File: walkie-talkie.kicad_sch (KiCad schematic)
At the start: 15 parts, among them J1 I2C, J2 Conn_01x08, J3 esp32-pico-kit, SW1 Transmit, SW2 POWER, U1 WARNING: Switch off when Plug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, U2 adafruit-MAX98357, U3 mems-mic

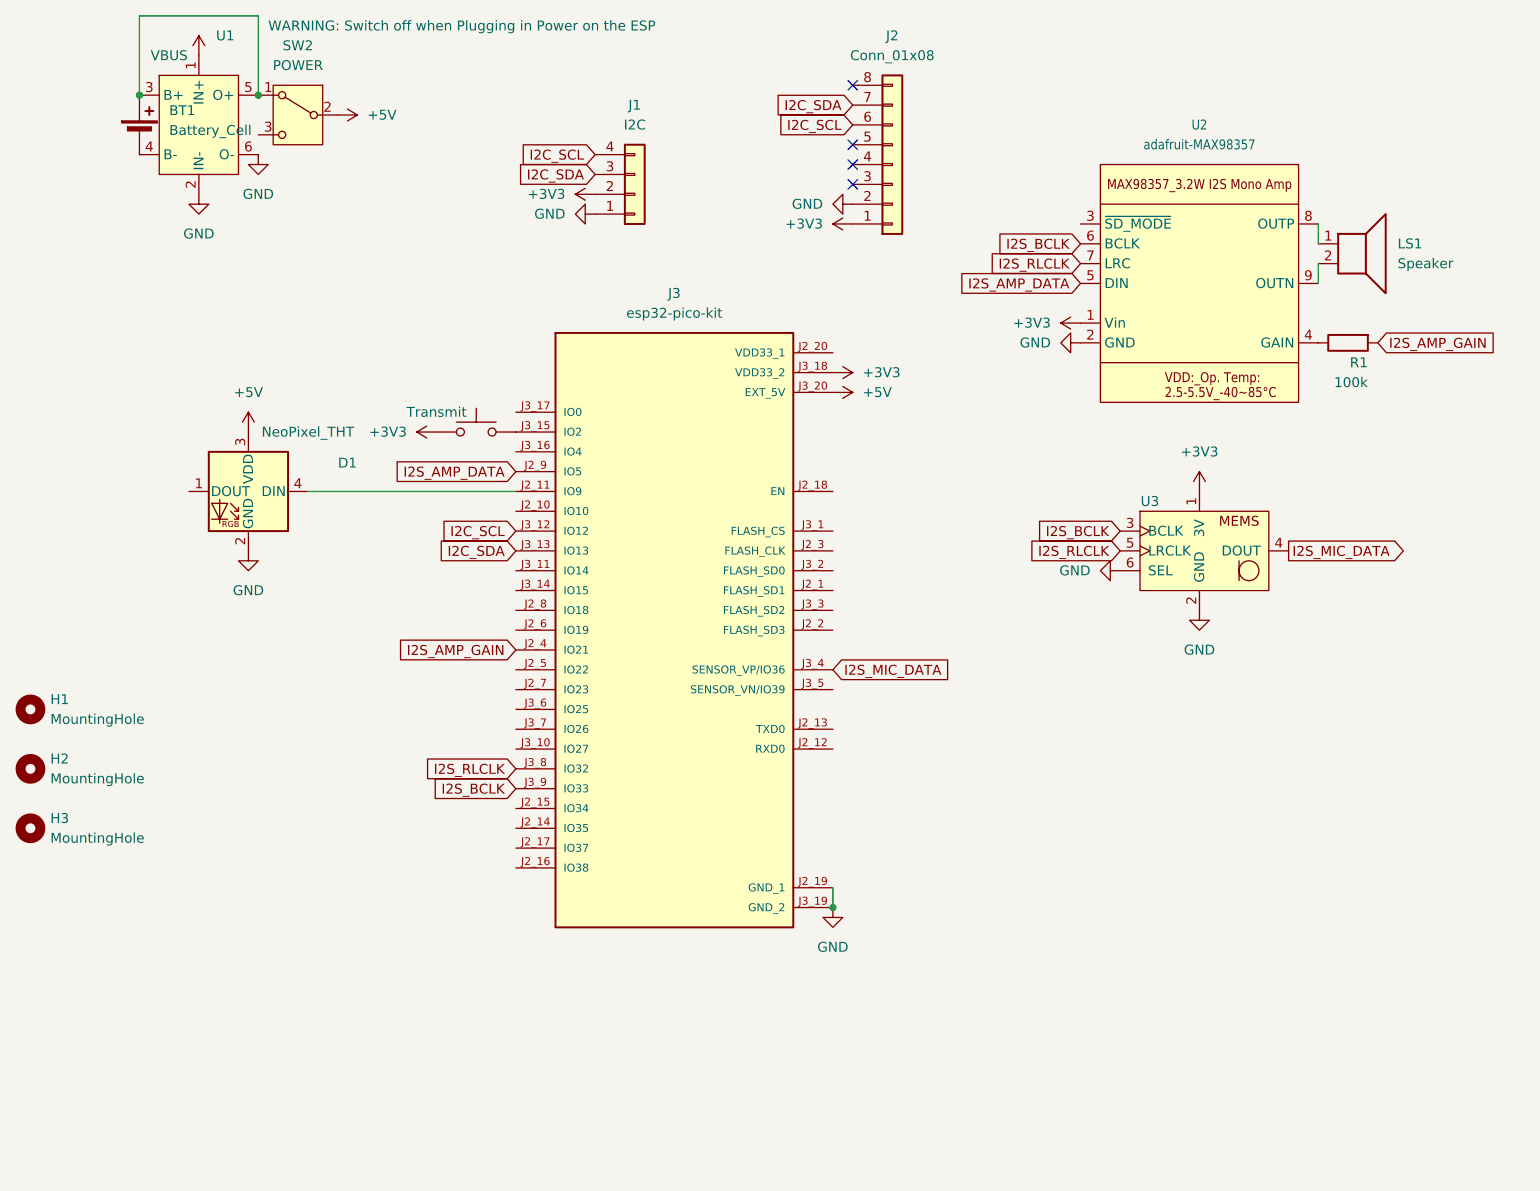
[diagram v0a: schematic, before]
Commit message: Lolin32-Lite PCB
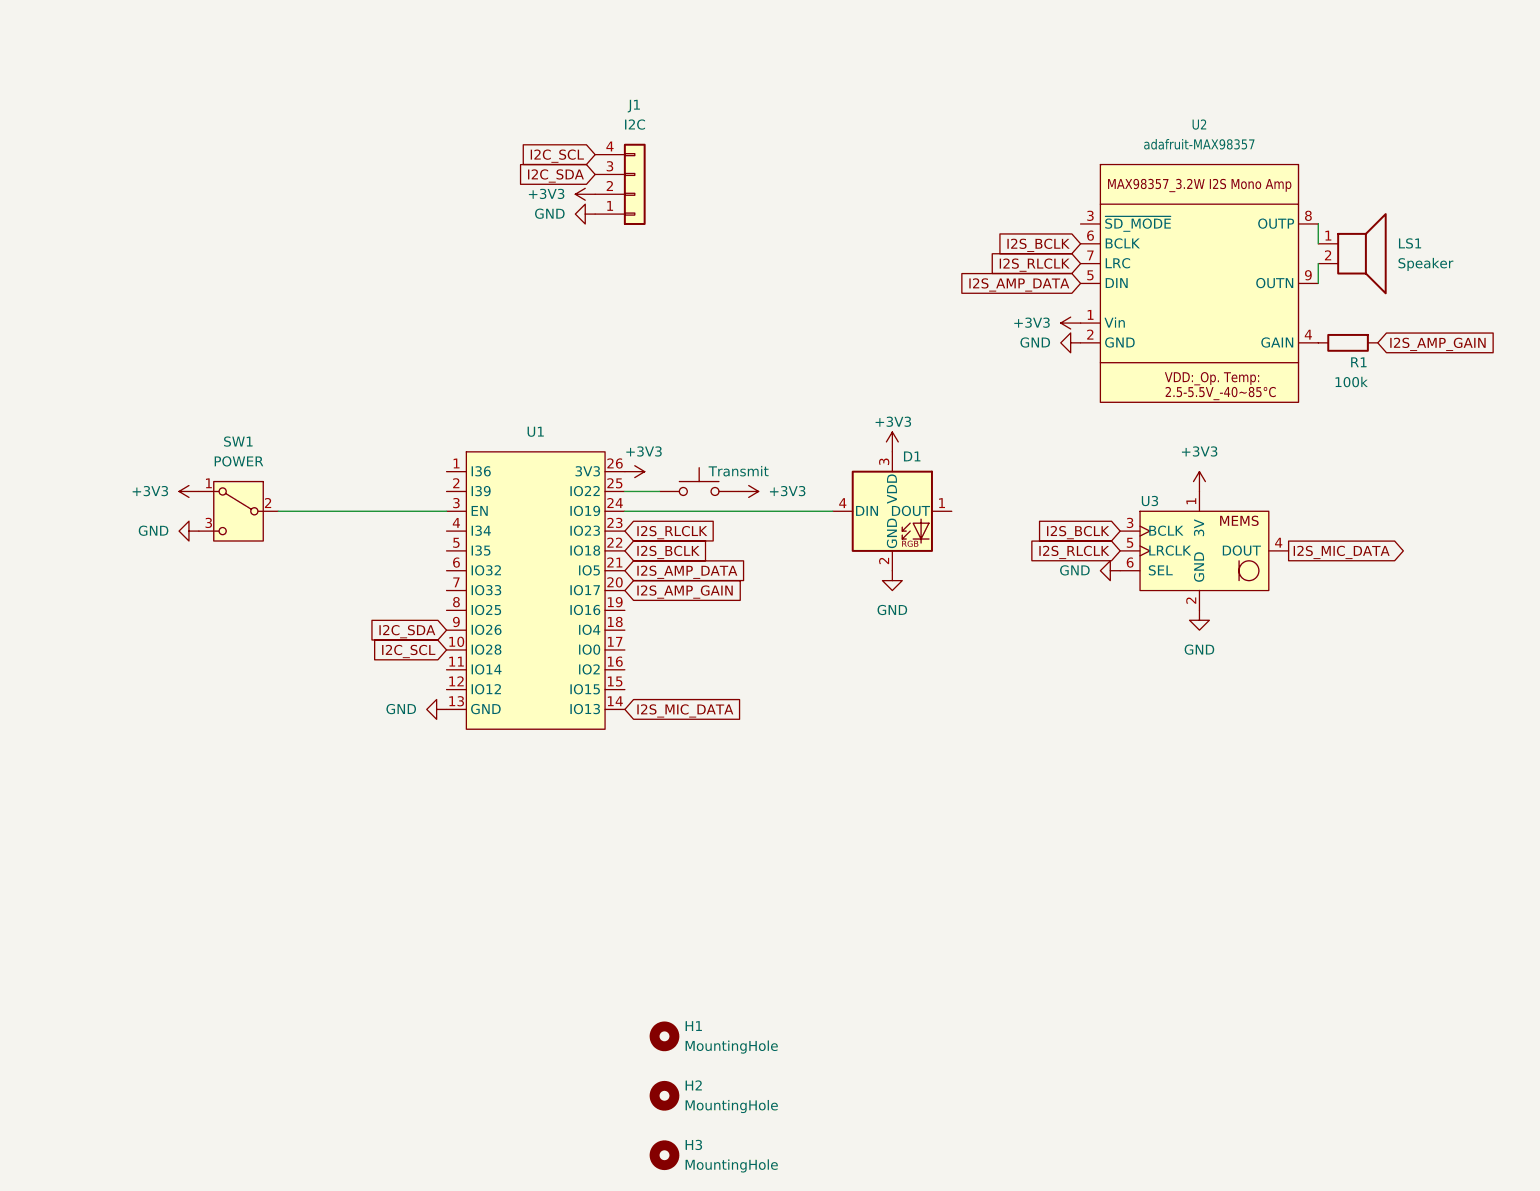
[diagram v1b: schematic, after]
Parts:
- removed BT1: Battery_Cell, Connector_JST:JST_XA_B02B-XASK-1_1x02_P2.50mm_Vertical, symbol Device:Battery_Cell
- removed J2: Conn_01x08, Connector_PinHeader_2.54mm:PinHeader_1x08_P2.54mm_Vertical, symbol Connector_Generic:Conn_01x08
- removed J3: esp32-pico-kit, esp32-pico-kit:esp32-pico-kit, symbol esp32-pico-kit:esp32-pico-kit
- removed SW1: Transmit, pts636:pts636, symbol Switch:SW_Push
- removed U1: WARNING: Switch off when Plugging in Power on the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, tp4056:tp4056, symbol tp4056:tp4056
- added SW2: Transmit, pts636:pts636, symbol Switch:SW_Push
- added U1: ~, lolin32-lite:lolin32-lite, symbol lolin32-lite:lolin32-lite
- renumbered SW2 to SW1
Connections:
- net +3V3: now also D1.3 (VDD), SW1.1 (A), SW2.2, U1.26 (3V3)
- net GND: now also SW1.3 (C), U1.13 (GND)
- net I2C_SCL: now also U1.10 (IO28)
- net I2C_SDA: now also U1.9 (IO26)
- net I2S_AMP_DATA: now also U1.21 (IO5)
- net I2S_AMP_GAIN: now also U1.20 (IO17)
- net I2S_BCLK: now also U1.22 (IO18)
- net I2S_MIC_DATA: now also U1.14 (IO13)
- net I2S_RLCLK: now also U1.23 (IO23)
- net at D1.4 (DIN): now also U1.24 (IO19)
- net +5V: no longer names the net of SW1.2 (B)
- net +5V: now also U1.3 (EN); no longer D1.3 (VDD)
- new net: SW2.1, U1.25 (IO22)
- no-connect marks 4 -> 0
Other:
- moved on the sheet: D1, H1, H2, H3, SW1
